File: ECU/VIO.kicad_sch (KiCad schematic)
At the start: 10 parts

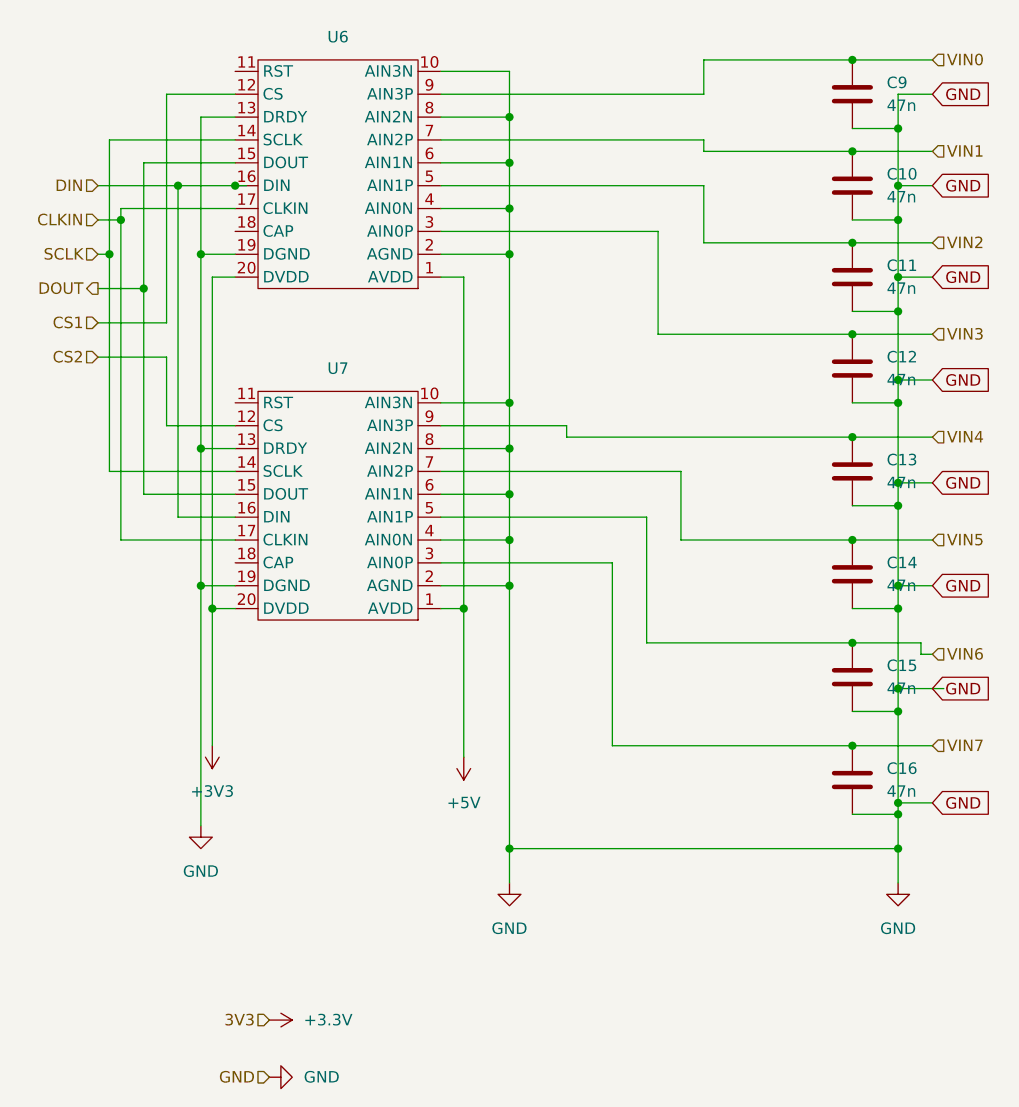
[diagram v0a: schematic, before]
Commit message: finished ECU
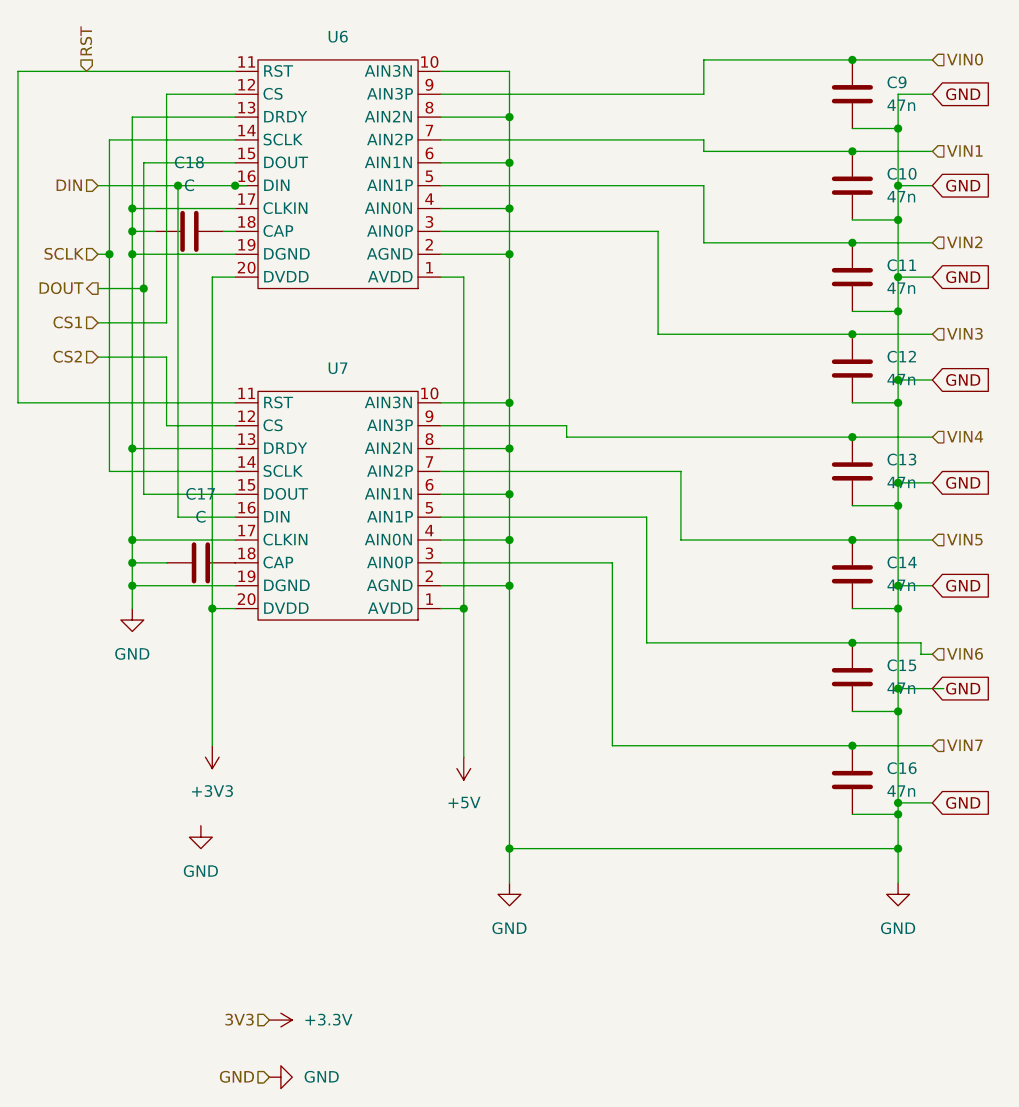
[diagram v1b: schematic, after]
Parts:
- added C17, C18: C, Capacitor_SMD:C_1206_3216Metric_Pad1.33x1.80mm_HandSolder, symbol Device:C
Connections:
- net CLKIN is gone; now on net GND: U6.17 (CLKIN), U7.17 (CLKIN)
- net GND: now also C17.2, C18.2
- net RST: now reaches U6.11 (RST)
- net RST: now also U7.11 (RST)
- net at U6.18 (CAP): now also C18.1
- net at U7.18 (CAP): now also C17.1
